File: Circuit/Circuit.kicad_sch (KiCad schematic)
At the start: 22 parts, among them SW1 SW_Push, SW10 SW_Push, SW11 SW_Push, SW12 SW_Push, SW13 SW_Push, SW14 SW_Push, SW15 SW_Push, SW16 SW_Push, SW17 SW_Push, SW18 SW_Push, SW19 SW_Push, SW2 SW_Push, SW20 SW_Push, SW21 SW_Push, SW3 SW_Push, SW4 SW_Push, SW5 SW_Push, SW6 SW_Push, SW7 SW_Push, SW8 SW_Push, SW9 SW_Push

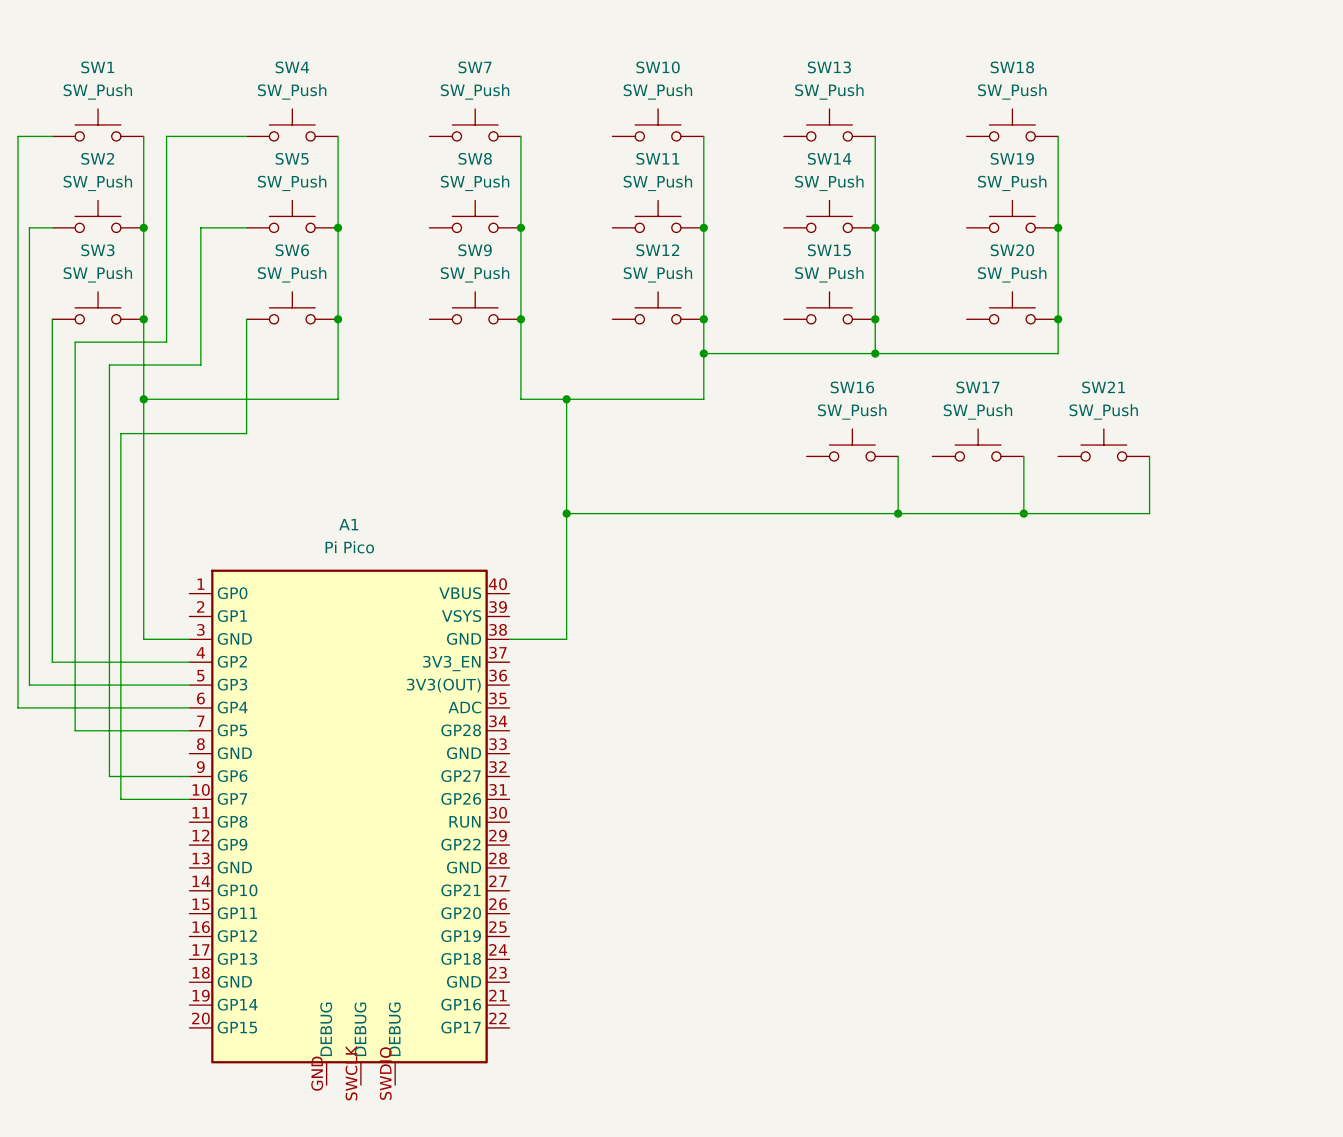
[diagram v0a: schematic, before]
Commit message: wiring
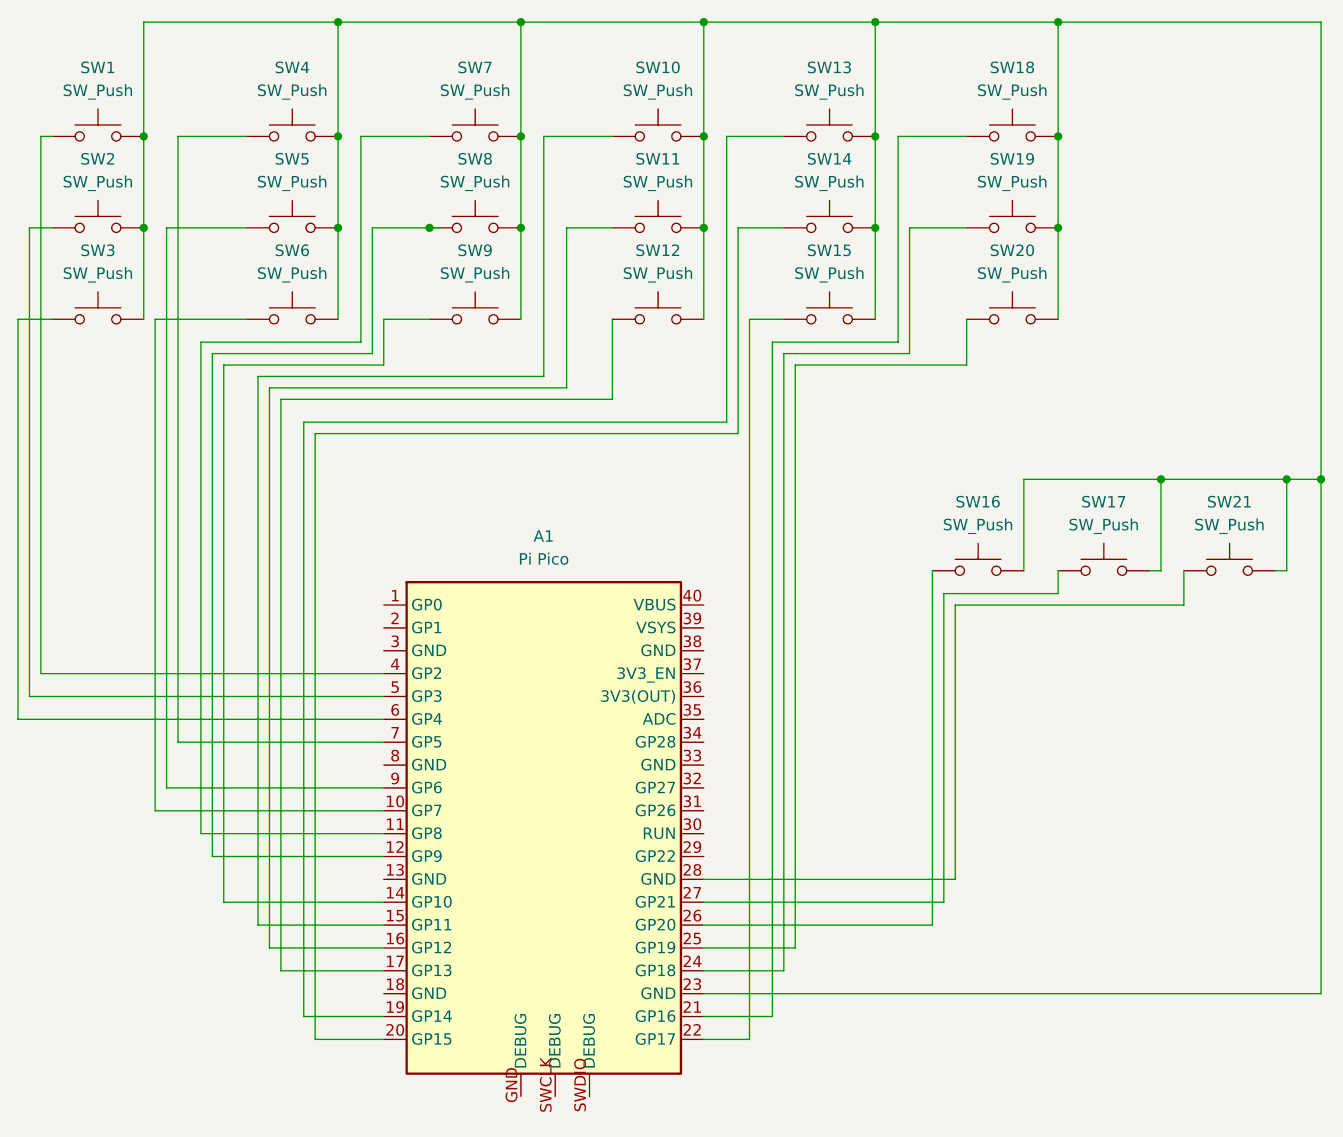
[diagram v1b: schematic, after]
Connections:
- net at SW12.1: now also A1.17 (GP13)
- net at SW10.2, SW11.2, SW12.2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: now also A1.23 (GND), SW1.2, SW2.2, SW3.2, SW4.2, SW5.2, SW6.2; no longer A1.38 (GND)
- net at SW11.1: now also A1.16 (GP12)
- net at SW10.1: now also A1.15 (GP11)
- net at SW7.1: now also A1.11 (GP8)
- net at SW15.1: now also A1.22 (GP17)
- net at SW21.1: now also A1.28 (GND)
- net at SW3.1: now also A1.6 (GP4); no longer A1.4 (GP2)
- net at SW20.1: now also A1.25 (GP19)
- net at SW8.1: now also A1.12 (GP9)
- net at SW1.1: now also A1.4 (GP2); no longer A1.6 (GP4)
- net at SW19.1: now also A1.24 (GP18)
- net at SW18.1: now also A1.21 (GP16)
- net at SW16.1: now also A1.26 (GP20)
- net at SW17.1: now also A1.27 (GP21)
- net at A1.14 (GP10): now also SW9.1
- net at A1.19 (GP14): now also SW13.1
- net at A1.20 (GP15): now also SW14.1
- now unconnected: A1.3 (GND)
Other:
- moved on the sheet: A1, SW16, SW17, SW21
